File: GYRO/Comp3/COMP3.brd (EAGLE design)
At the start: 35.5 x 18.7 mm, 21 parts, among them U2 LSM9DS1

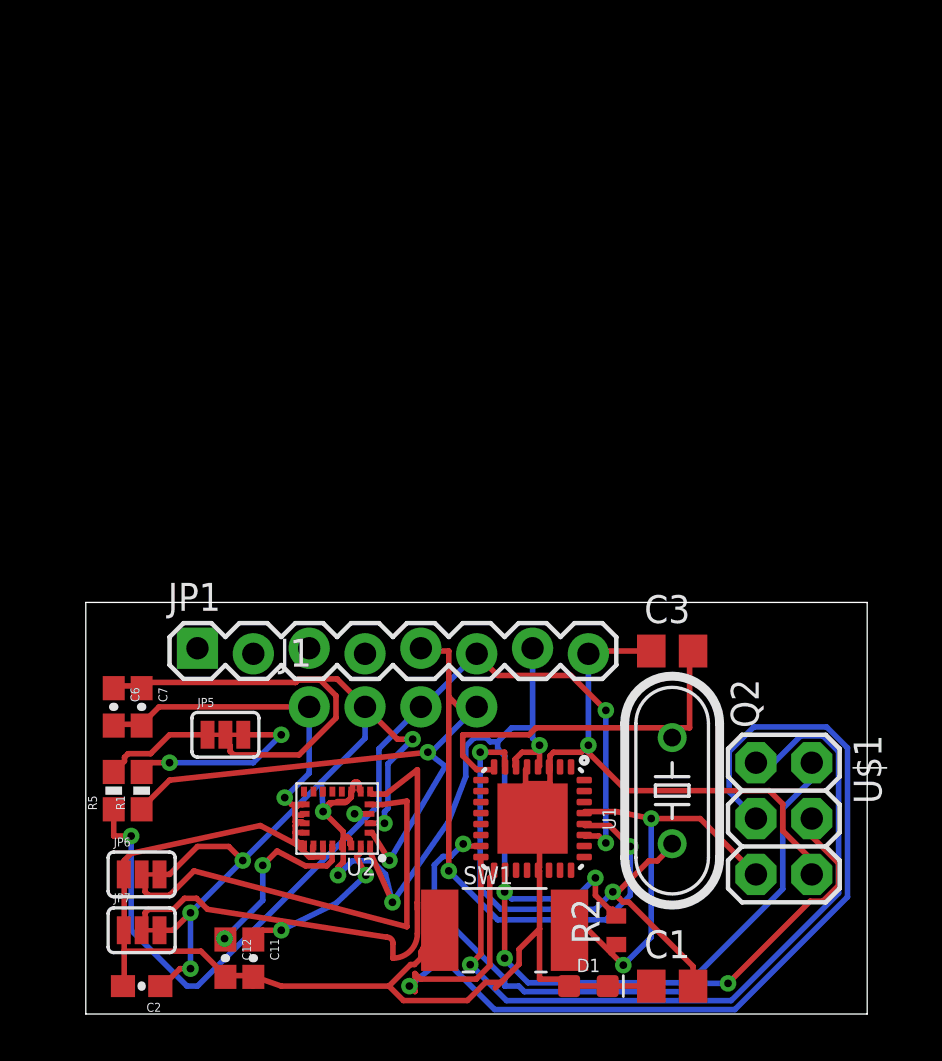
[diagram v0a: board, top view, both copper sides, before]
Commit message: Revert "s"
This reverts commit f00e3bdaf57eb9e1bba398a63e28bb58f9eab196.
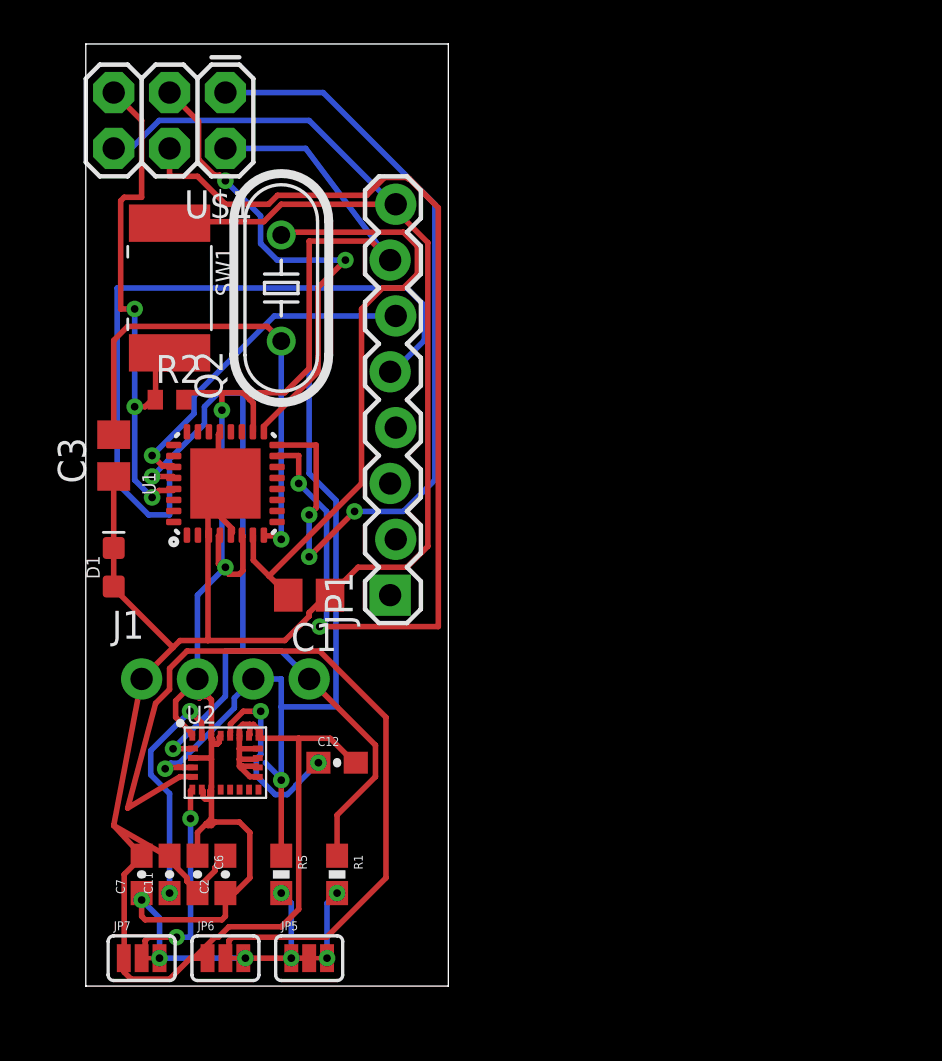
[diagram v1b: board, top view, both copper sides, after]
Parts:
- moved U$1 38.9 mm to (6.35, 41.9), turned to 180 degrees
- moved SW1 32.9 mm to (3.81, 33.0), turned to 270 degrees
- moved R2 31.5 mm to (3.81, 27.9), turned to 0 degrees
- moved Q2 29.0 mm to (8.89, 33.0), turned to 90 degrees
- moved D1 28.8 mm to (1.27, 20.3), turned to 90 degrees
- moved C3 26.9 mm to (1.27, 25.4), turned to 90 degrees
- moved C1 24.3 mm to (10.2, 19.1), turned to 180 degrees
- moved U1 20.7 mm to (6.35, 24.1), turned to 90 degrees
- moved JP5 10.9 mm to (10.2, 2.54)
- moved C12 10.2 mm to (11.4, 11.4), turned to 0 degrees
- moved R1 9.67 mm to (11.4, 6.35), turned to 270 degrees
- moved JP1 9.25 mm to (14.0, 19.1), turned to 90 degrees
- moved C6 8.52 mm to (5.08, 6.35)
- moved R5 8.52 mm to (8.89, 6.35), turned to 270 degrees
- moved J1 7.73 mm to (2.54, 15.2)
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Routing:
- net VCC: track 128.4 -> 83.3 mm, vias 12 -> 5
- net GND: track 103.9 -> 132.1 mm, vias 2 -> 0
- net SCK: track 49.4 -> 22.2 mm, vias 1 -> 2
- net SCL: track 51.6 -> 72.0 mm, vias 4 -> 2
- net MOSI: track 30.2 -> 49.1 mm
- net SDO_A/G: track 21.1 -> 38.1 mm
- net SDO_M: track 25.5 -> 9.84 mm, vias 0 -> 2
- net SDA: track 46.2 -> 53.8 mm, vias 4 -> 3
- net N$2: track 8.78 -> 3.15 mm
- net RESET: track 19.9 -> 25.4 mm, vias 2 -> 3
- net N$3: track 17.6 -> 22.4 mm, vias 0 -> 1
- net N$4: track 24.8 -> 28.3 mm, vias 2 -> 0
- net N$6: track 7.62 -> 10.7 mm
- net MISO: track 35.6 -> 38.3 mm, vias 1 -> 3
- net N$1: track 5.07 -> 3.15 mm, vias 0 -> 2
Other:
- board size 35.5 x 18.7 mm -> 16.5 x 42.8 mm
